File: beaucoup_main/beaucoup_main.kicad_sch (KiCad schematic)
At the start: 21 parts, among them J1 RGBled, J10 Conn_01x03_Pin, J11 AMP, J12 tomist, J2 NFCreader, J3 potenziometro, J5 conn_bottone_mist, J6 Conn_01x02_Pin, J7 Conn_01x02_Pin, J8 Conn_01x02_Pin, J9 Conn_01x02_Pin, Q1 2N7002, U1 rp2040_XIAO, U2 DFPlayer

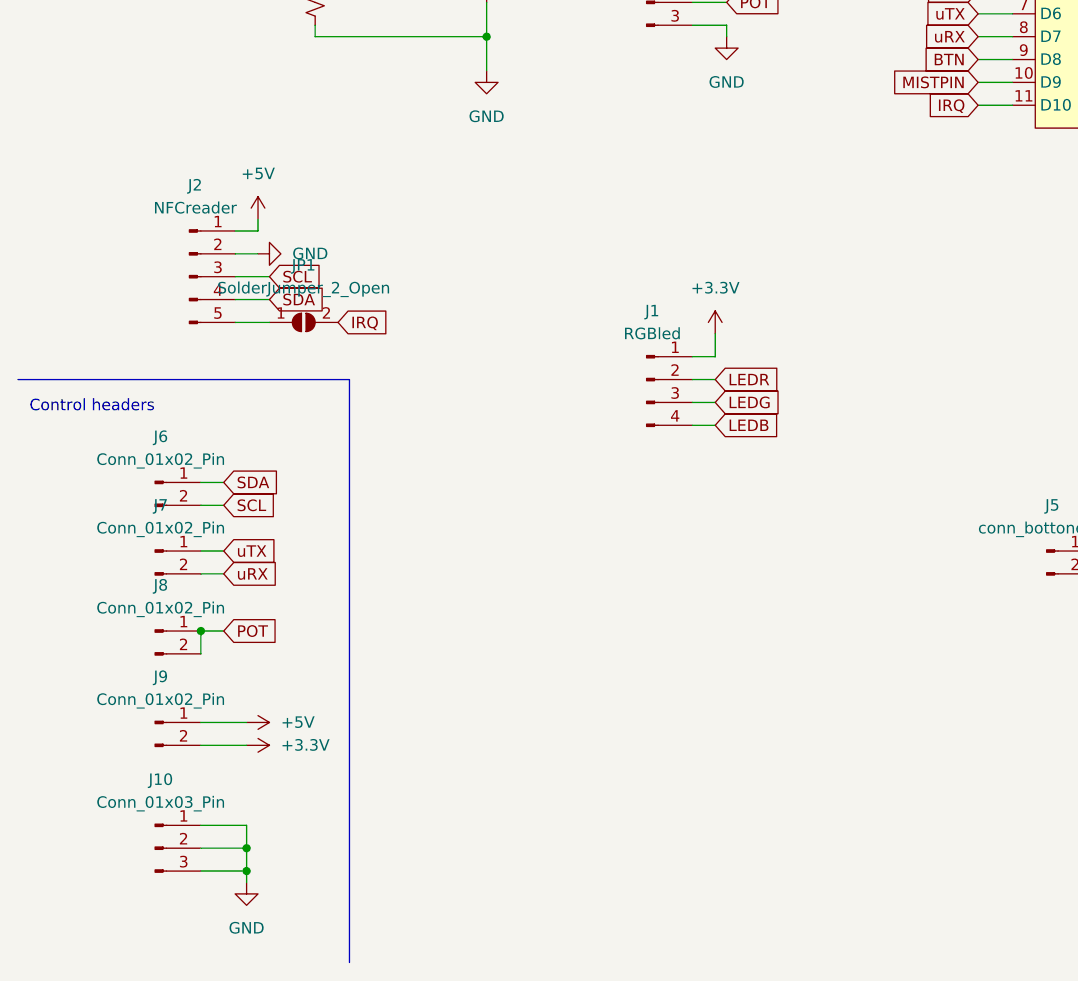
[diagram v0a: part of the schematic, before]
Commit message: Main pcb should be ready for production
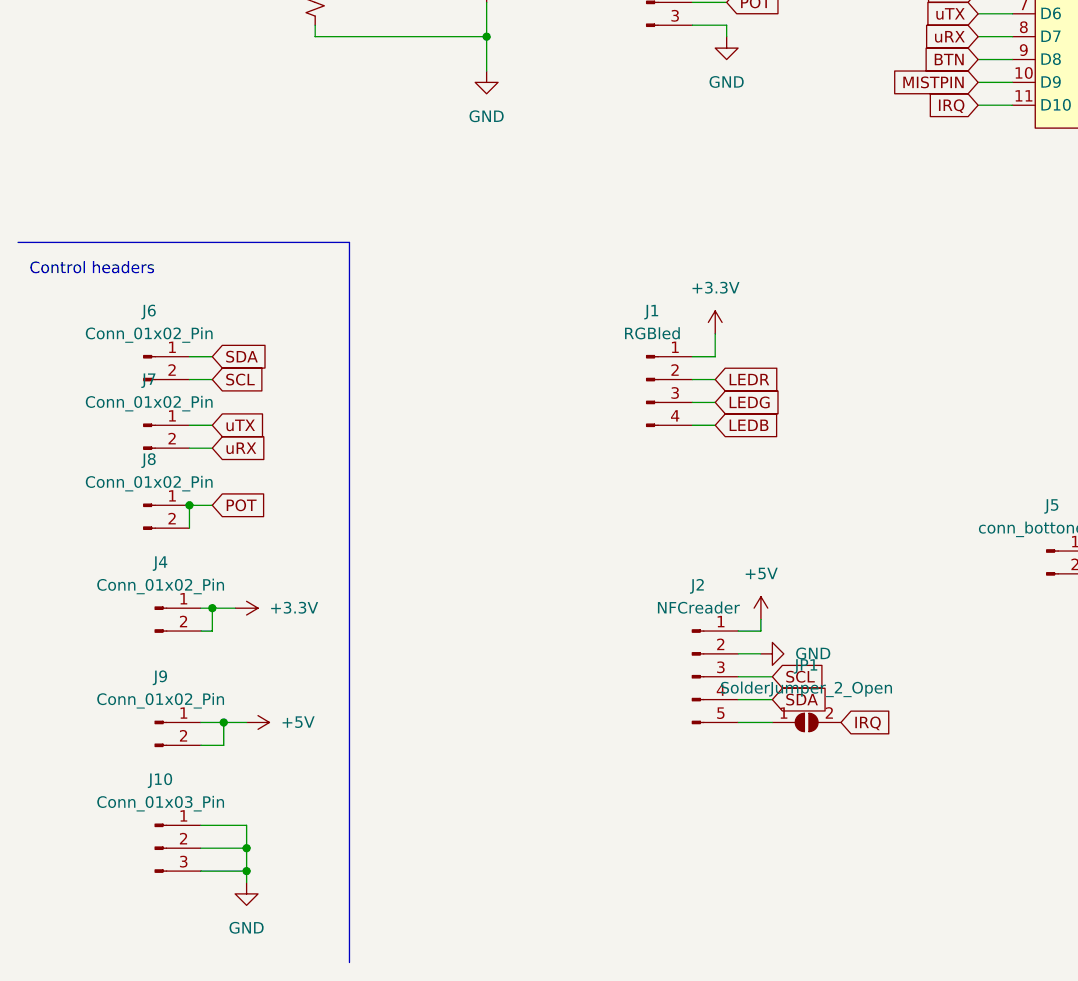
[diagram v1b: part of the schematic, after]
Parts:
- added J4: Conn_01x02_Pin, Connector_PinHeader_2.54mm:PinHeader_1x02_P2.54mm_Vertical, symbol Connector:Conn_01x02_Pin
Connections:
- net +3.3V: now also J4.1 (Pin_1), J4.2 (Pin_2); no longer J9.2 (Pin_2)
- net +5V: now also J9.2 (Pin_2)
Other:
- moved on the sheet: J2, J6, J7, J8, JP1
